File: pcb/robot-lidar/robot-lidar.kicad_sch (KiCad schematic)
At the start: 1 part, among them U1 STM32F429VETx

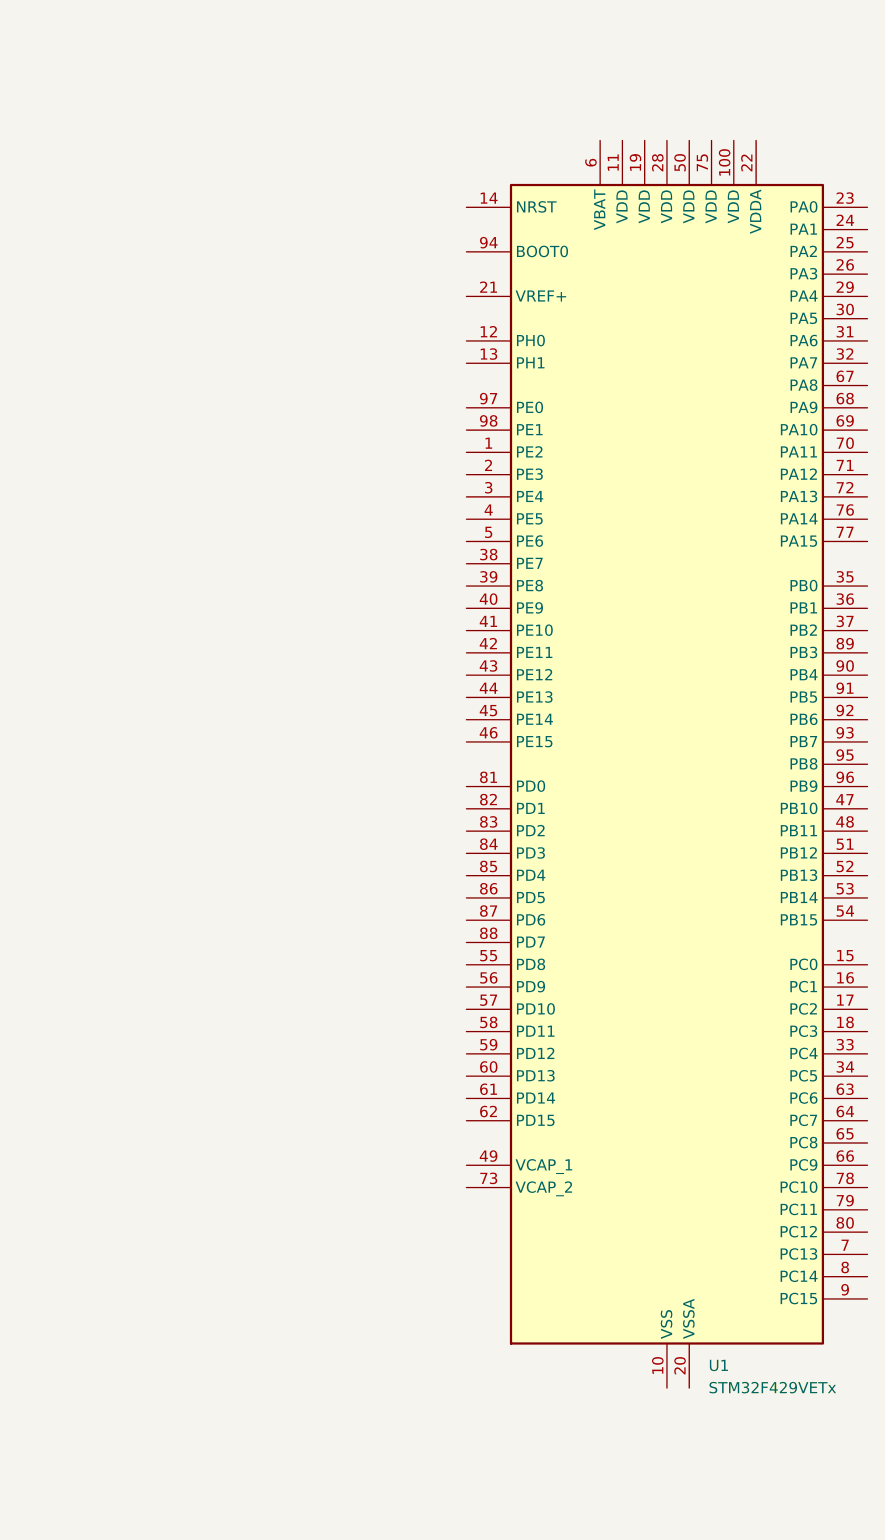
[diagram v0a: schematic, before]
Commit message: add jack
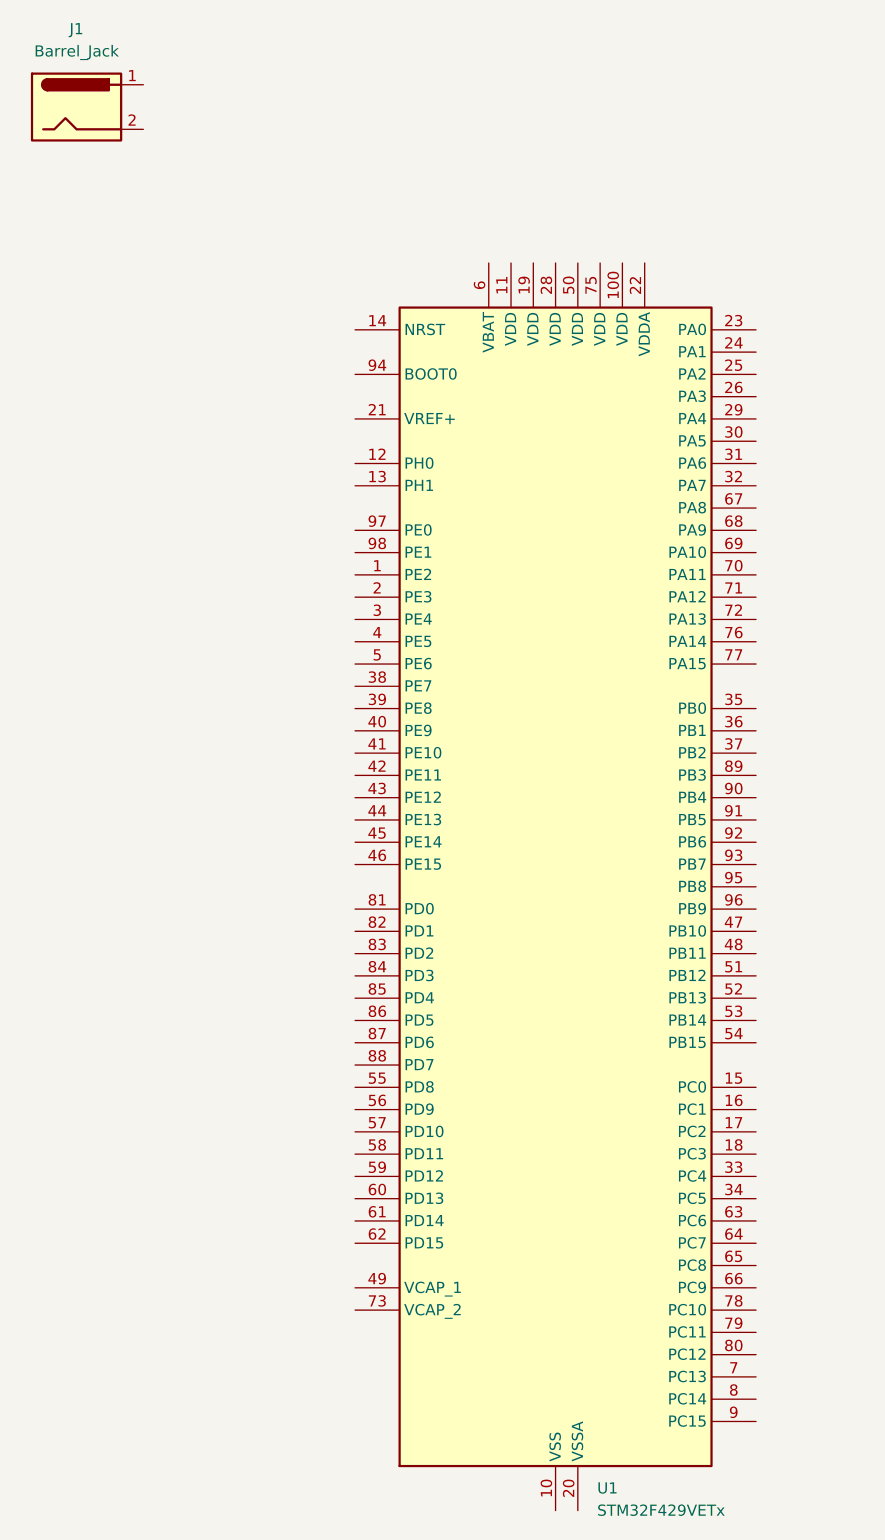
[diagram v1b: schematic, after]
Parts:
- added J1: Barrel_Jack, symbol Connector:Barrel_Jack
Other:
- moved on the sheet: U1
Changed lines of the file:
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@@
 (kicad_sch (version 20230121) (generator eeschema)
   (paper "A4")
-  (symbol (lib_id "MCU_ST_STM32F4:STM32F429VETx") (at 90.17 99.06 0) (unit 1)
+  (symbol (lib_id "MCU_ST_STM32F4:STM32F429VETx") (at 77.47 113.03 0) (unit 1)
     (in_bom yes) (on_board yes) (dnp no) (fields_autoplaced)
-    (property "Reference" "U1" (at 94.9041 167.64 0)
+    (property "Reference" "U1" (at 82.2041 181.61 0)
       (effects (font (size 1.27 1.27)) (justify left))
     )
-    (property "Value" "STM32F429VETx" (at 94.9041 170.18 0)
+    (property "Value" "STM32F429VETx" (at 82.2041 184.15 0)
       (effects (font (size 1.27 1.27)) (justify left))
     )
-    (property "Footprint" "Package_QFP:LQFP-100_14x14mm_P0.5mm" (at 72.39 165.1 0)
+    (property "Footprint" "Package_QFP:LQFP-100_14x14mm_P0.5mm" (at 59.69 179.07 0)
       (effects (font (size 1.27 1.27)) (justify right) hide)
     )
-    (property "Datasheet" "https://www.st.com/resource/en/datasheet/stm32f429ve.pdf" (at 90.17 99.06 0)
+    (property "Datasheet" "https://www.st.com/resource/en/datasheet/stm32f429ve.pdf" (at 77.47 113.03 0)
       (effects (font (size 1.27 1.27)) hide)
     )
@@
         )
       )
+    )
+  )
+  (symbol (lib_id "Connector:Barrel_Jack") (at 22.86 24.13 0) (unit 1)
+    (in_bom yes) (on_board yes) (dnp no) (fields_autoplaced)
+    (property "Reference" "J1" (at 22.86 15.24 0)
+      (effects (font (size 1.27 1.27)))
+    )
+    (property "Value" "Barrel_Jack" (at 22.86 17.78 0)
+      (effects (font (size 1.27 1.27)))
+    )
+    (property "Footprint" "" (at 24.13 25.146 0)
+      (effects (font (size 1.27 1.27)) hide)
+    )
+    (property "Datasheet" "~" (at 24.13 25.146 0)
+      (effects (font (size 1.27 1.27)) hide)
+    )
+    (pin "1")
+    (pin "2")
+    (instances
+      (project "robot-lidar"
+        (path "/cb10bbf7-c2c1-4a0d-8947-ad707931d83b"
+          (reference "J1") (unit 1)
+        )
+      )
